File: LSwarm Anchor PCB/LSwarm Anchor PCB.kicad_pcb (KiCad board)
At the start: 4 copper layers, 82.5 x 28 mm, 56 parts, among them Q7 AO3407A, SW1 MSK12C02, U1 BQ24075RGTR, U12 AP2112K-3.3, U2 BU03, U4 DW03C_C41367942, U6 ESP32-C3-MINI-1U-N4

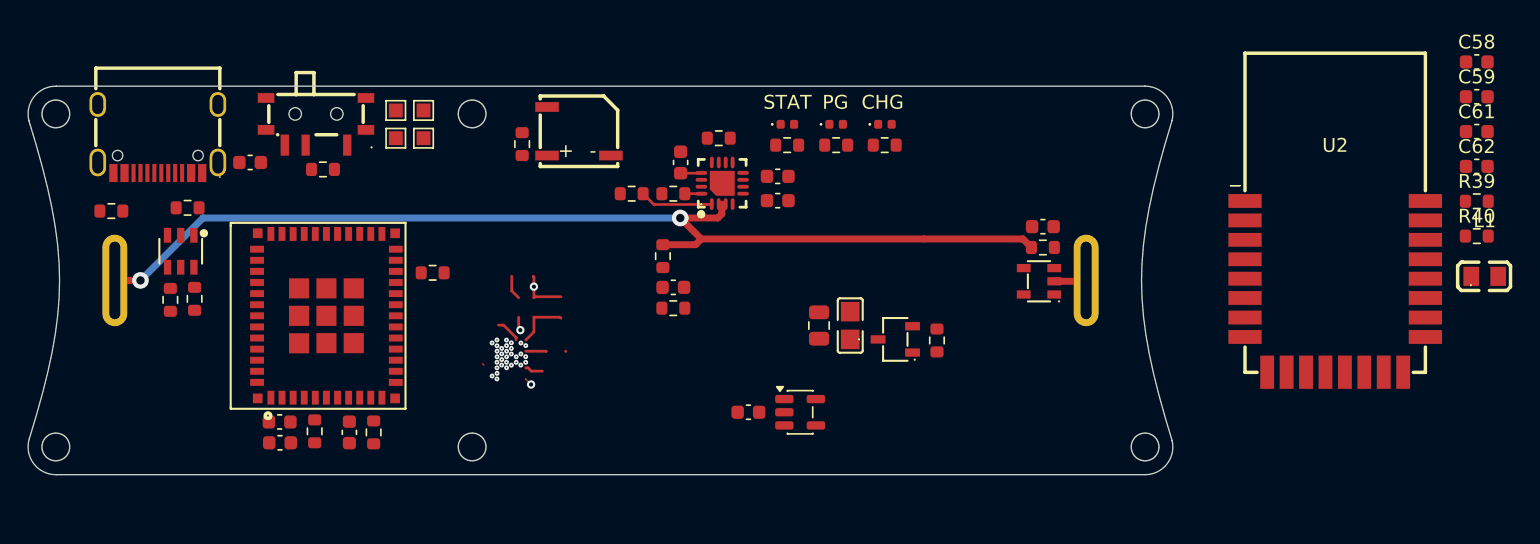
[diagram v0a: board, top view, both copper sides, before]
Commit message: sync
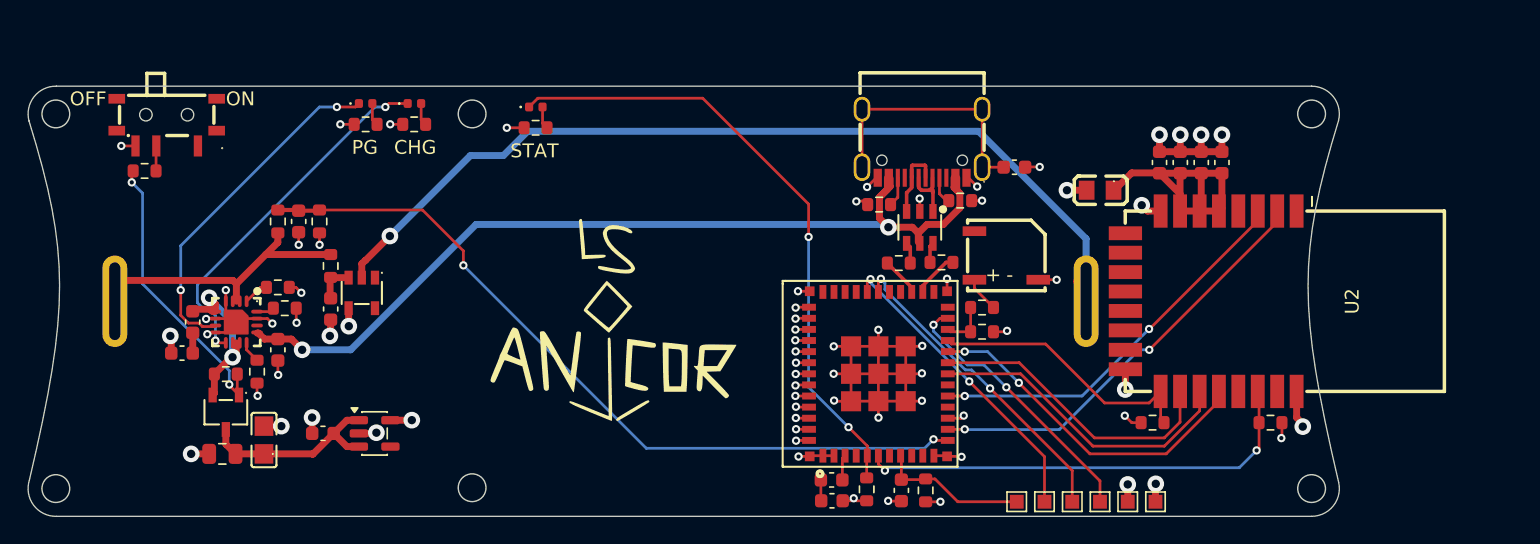
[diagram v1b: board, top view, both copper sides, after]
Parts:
- added G***: LOGO, LOGO, F.Cu at (40.5, 26.7)
- added TP39: 3.3V REF, TestPoint:TestPoint_Pad_1.0x1.0mm, F.Cu at (81.2, 29.9)
- added TP41: GND REF, TestPoint:TestPoint_Pad_1.0x1.0mm, F.Cu at (79.2, 29.9)
- moved TP36 57.1 mm to (77.2, 29.9)
- moved R37 55.7 mm to (67.2, 8.25)
- moved R34 55.3 mm to (61.3, 8.53)
- moved USB1 55.1 mm to (64.4, 4.13)
- moved C27 55.1 mm to (71.1, 5.84)
- moved TP38 54.6 mm to (75.2, 29.9)
- moved TP40 54.6 mm to (73.2, 29.9)
- moved R35 53.9 mm to (65.8, 12.7), turned to 0 degrees
- moved D5 53.3 mm to (64.3, 10.2)
- moved R36 52.6 mm to (62.8, 12.8), turned to 0 degrees
- moved C31 51.7 mm to (21.8, 16.1), turned to -90 degrees
- moved R16 51.3 mm to (21.8, 13.0), turned to -90 degrees
- moved R28 51.3 mm to (14.2, 20.8), turned to 180 degrees
- moved TP34 50.1 mm to (71.2, 29.9)
- moved U4 48.8 mm to (24.1, 14.9), turned to 180 degrees
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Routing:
- net GND: track 5.09 -> 105.5 mm, vias 27 -> 61
- net USB_VBUS: track 1.51 -> 66.1 mm, vias 0 -> 2
- net BATT-: track 2.32 -> 65.6 mm, vias 0 -> 1
- net ESP32_VMON_ADC: track 0.00 -> 56.3 mm, vias 0 -> 2
- net BATT+: track 75.6 -> 20.2 mm, vias 2 -> 0
- net ESP32_STATUS: track 0.00 -> 45.1 mm, vias 0 -> 2
- net DW_IRQ: track 0.00 -> 33.0 mm, vias 1 -> 2
- net DW_WAKEUP: track 0.00 -> 30.7 mm, vias 1 -> 2
- net DW_RST: track 0.00 -> 28.3 mm, vias 0 -> 2
- net Net-(D7-K): track 0.00 -> 26.2 mm, vias 0 -> 2
- net Net-(D8-K): track 0.00 -> 25.0 mm, vias 0 -> 2
- net DW_CLK: track 0.00 -> 24.2 mm, vias 0 -> 2
- net Net-(U6-RXD0): track 0.00 -> 23.1 mm, vias 0 -> 2
- net UW_3.3V: track 0.00 -> 22.8 mm
- net DW_MISO: track 0.14 -> 22.8 mm
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- added copper zone on In2.Cu, net +3.3V
- added copper zone on In1.Cu, net GND
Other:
- board size 82.5 x 28 mm -> 94.5 x 31 mm
- board text added: "OFF"
- board text added: "ON"
